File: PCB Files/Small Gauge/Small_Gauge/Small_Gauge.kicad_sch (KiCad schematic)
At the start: 30 parts, among them J1 USB_B_Micro, J2 Conn_01x02, J3 Conn_02x18_Odd_Even, J4 Conn_02x18_Odd_Even, U1 RP2040, U2 NCP1117-3.3_SOT223, U3 W25Q128JVS, Y1 ABM8G-12.000MHZ-18-D2Y-T3

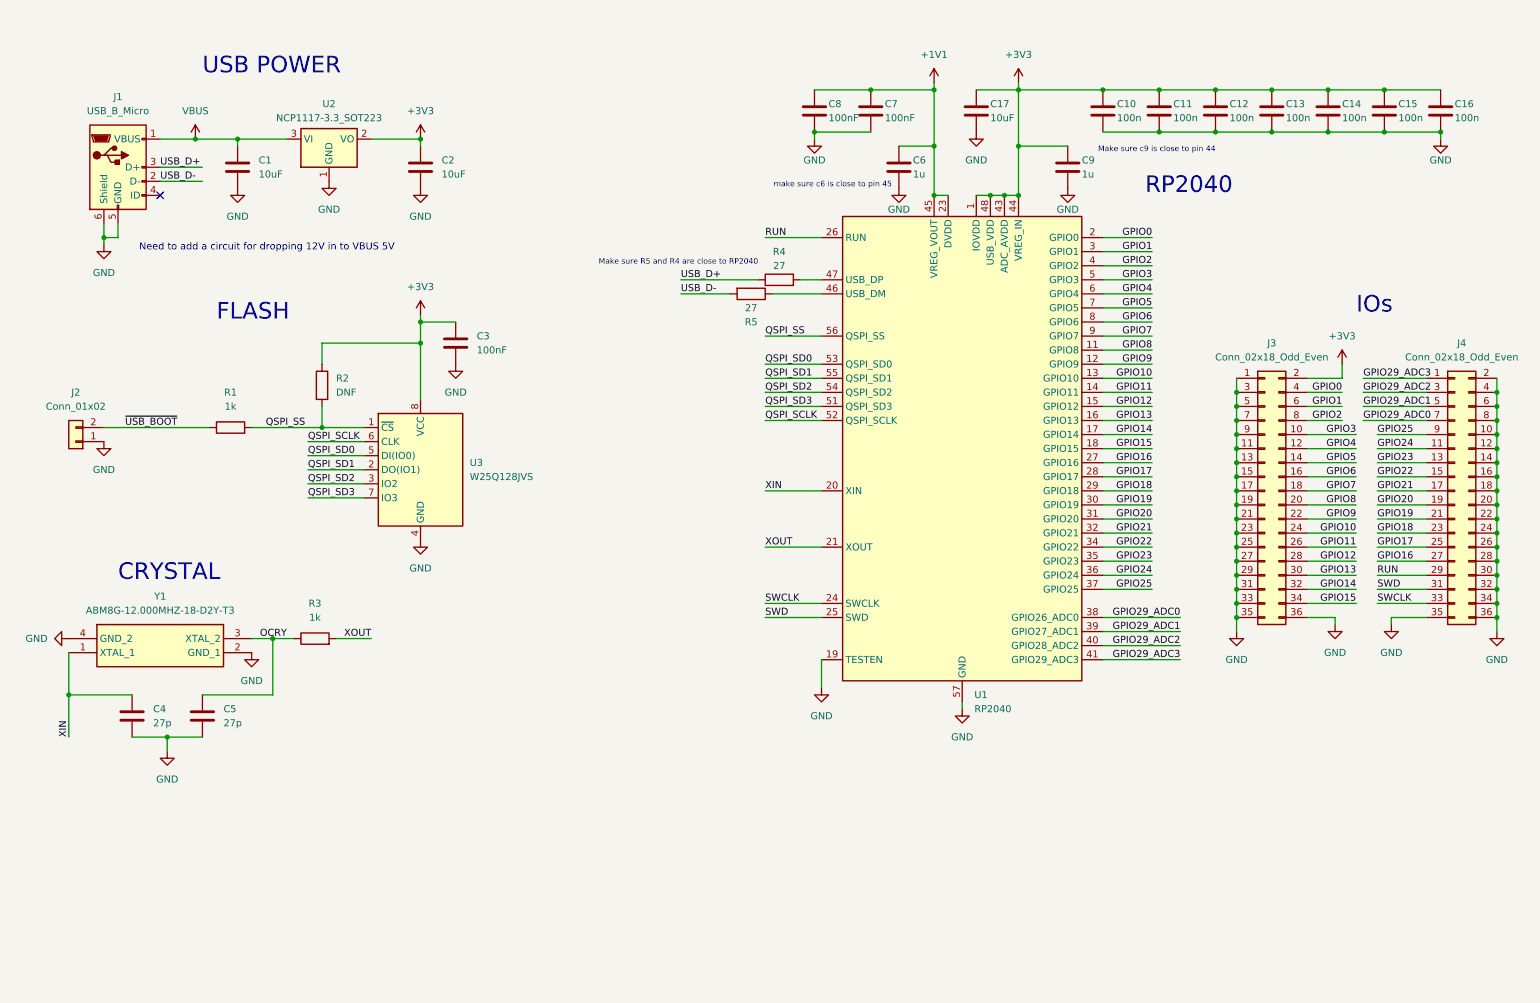
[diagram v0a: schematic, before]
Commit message: KiCad ESP 32 stuff
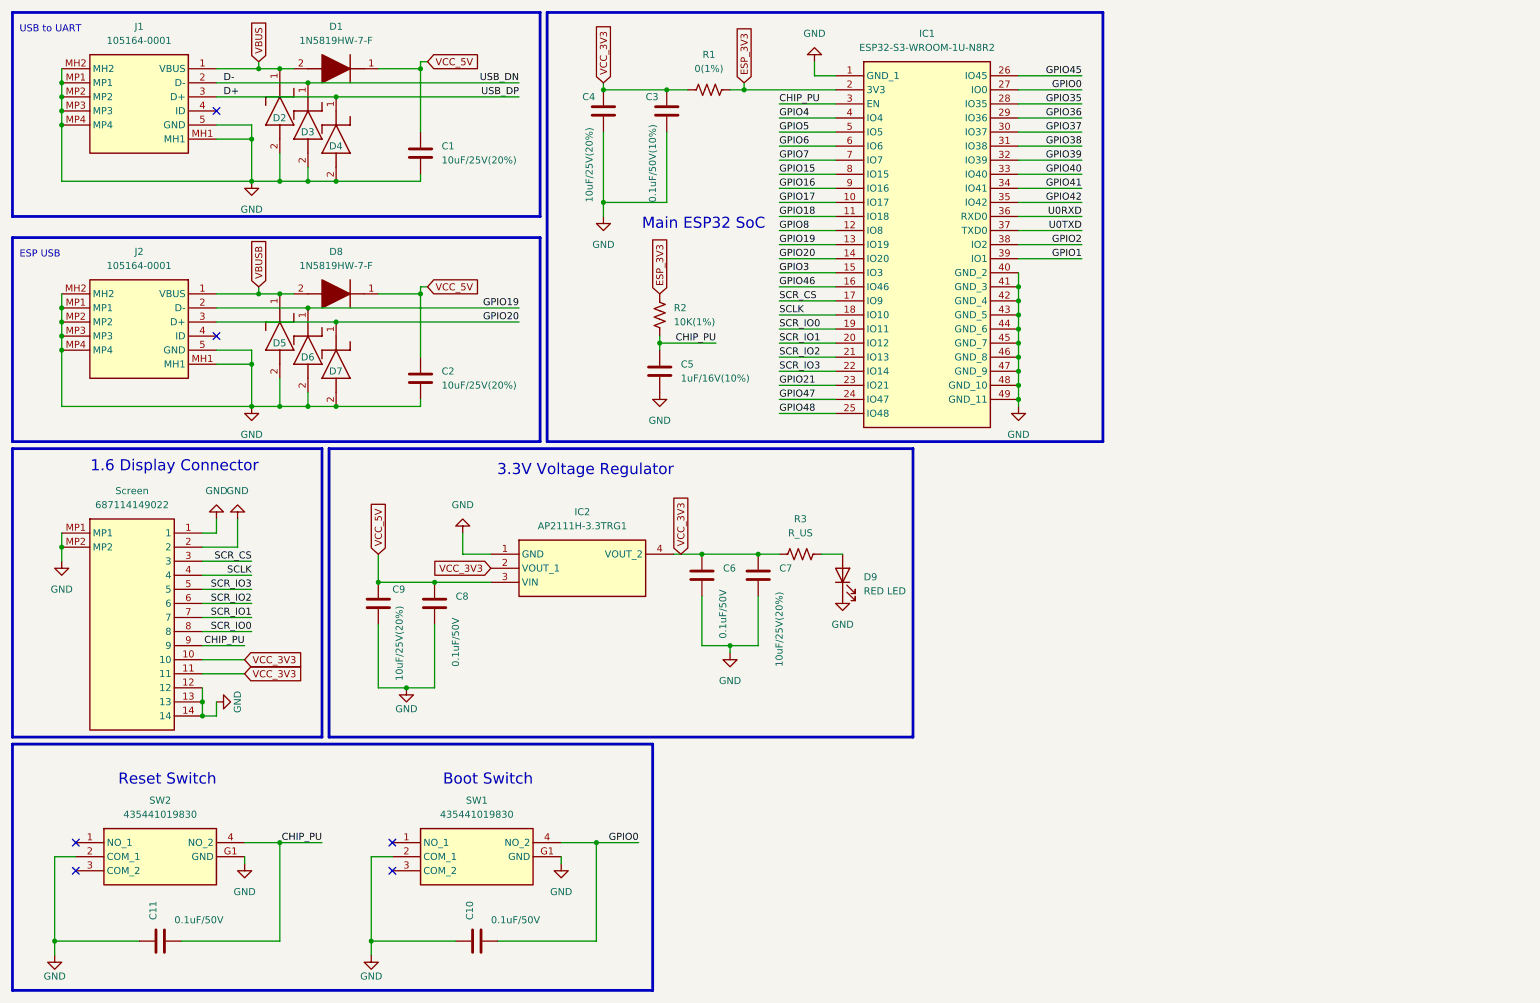
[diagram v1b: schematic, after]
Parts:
- removed C12, C13, C14, C15, C16: 100n, Resistor_SMD:R_0201_0603Metric, symbol Device:C
- removed C17: 10uF, Capacitor_SMD:C_0402_1005Metric_Pad0.74x0.62mm_HandSolder, symbol Device:C
- removed J1: USB_B_Micro, Mouser:USB_MICRO_B_1051640001, symbol Connector:USB_B_Micro
- removed J2: Conn_01x02, Connector_JST:JST_EH_B2B-EH-A_1x02_P2.50mm_Vertical, symbol Connector_Generic:Conn_01x02
- removed J3, J4: Conn_02x18_Odd_Even, Connector_JST:JST_PUD_B36B-PUDSS_2x18_P2.00mm_Vertical, symbol Connector_Generic:Conn_02x18_Odd_Even
- removed R1, R3: 1k, Resistor_SMD:R_0201_0603Metric_Pad0.64x0.40mm_HandSolder, symbol Device:R
- removed R2: DNF, Resistor_SMD:R_0201_0603Metric_Pad0.64x0.40mm_HandSolder, symbol Device:R
- removed R4, R5: 27, Resistor_SMD:R_0402_1005Metric, symbol Device:R
- removed U1: RP2040, Package_DFN_QFN:QFN-56-1EP_7x7mm_P0.4mm_EP3.2x3.2mm, symbol MCU_RaspberryPi:RP2040
- removed U2: NCP1117-3.3_SOT223, Package_TO_SOT_SMD:SOT-223-3_TabPin2, symbol Regulator_Linear:NCP1117-3.3_SOT223
- removed U3: W25Q128JVS, Package_SO:SOIC-8_5.23x5.23mm_P1.27mm, symbol Memory_Flash:W25Q128JVS
- removed Y1: ABM8G-12.000MHZ-18-D2Y-T3, Mouser:ABM8G, symbol ABM8G-12_000MHZ-18-D2Y-T3:ABM8G-12.000MHZ-18-D2Y-T3
- added D1, D8: 1N5819HW-7-F, SOD3716X145N, symbol SamacSys_Parts:1N5819HW-7-F
- added D2, D3, D4, D5, D6, D7: ESDA7P60-1U1M, ESDA7P601U1M, symbol SamacSys_Parts:ESDA7P60-1U1M
- added D9: RED LED, Resistor_SMD:R_1206_3216Metric_Pad1.30x1.75mm_HandSolder, symbol Device:LED
- added IC1: ESP32-S3-WROOM-1U-N8R2, ESP32S3WROOM1UN8R2, symbol SamacSys_Parts:ESP32-S3-WROOM-1U-N8R2
- added IC2: AP2111H-3.3TRG1, SOT230P700X180-4N, symbol SamacSys_Parts:AP2111H-3.3TRG1
- added J1, J2: 105164-0001, 1051640001, symbol SamacSys_Parts:105164-0001
- added R1: 0(1%), Resistor_SMD:R_0603_1608Metric_Pad0.98x0.95mm_HandSolder, symbol Device:R_US
- added R2: 10K(1%), Resistor_SMD:R_1206_3216Metric, symbol Device:R_US
- added R3: R_US, Resistor_SMD:R_1206_3216Metric, symbol Device:R_US
- added SW1, SW2: 435441019830, SamacSys_Parts:435441019830, symbol SamacSys_Parts:435441019830
- added Screen: 687114149022, 687114149022, symbol SamacSys_Parts:687114149022
- C1, C2: value 10uF -> 10uF/25V(20%); footprint Capacitor_SMD:C_0402_1005Metric_Pad0.74x0.62mm_HandSolder -> Capacitor_SMD:C_1206_3216Metric; Price 0.27 -> (none); Vendor https://www.mouser.com/ProductDetail/KYOCERA-AVX/04026D106M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 -> (none)
- C10, C11: value 100n -> 0.1uF/50V; footprint Resistor_SMD:R_0201_0603Metric -> Resistor_SMD:R_1206_3216Metric; Price 0.10 -> (none); Vendor https://www.mouser.com/ProductDetail/TDK/C0603X5R1E104K030B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 -> (none)
- C3: value 100nF -> 0.1uF/50V(10%); footprint Resistor_SMD:R_0201_0603Metric -> (none); Price 0.10 -> (none); Vendor https://www.mouser.com/ProductDetail/TDK/C0603X5R1E104K030B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 -> (none)
- C4: value 27p -> 10uF/25V(20%); footprint Capacitor_SMD:C_0201_0603Metric -> (none); Price 0.10 -> (none); Vendor https://www.mouser.com/ProductDetail/Murata-Electronics/GRT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 -> (none)
- C5: value 27p -> 1uF/16V(10%); footprint Capacitor_SMD:C_0201_0603Metric -> Resistor_SMD:R_1206_3216Metric; Price 0.10 -> (none); Vendor https://www.mouser.com/ProductDetail/Murata-Electronics/GRT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 -> (none)
- C6: value 1u -> 0.1uF/50V; footprint Capacitor_SMD:C_0201_0603Metric -> Resistor_SMD:R_1206_3216Metric; Price 0.12 -> (none); Vendor https://www.mouser.com/ProductDetail/KYOCERA-AVX/02016D105M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 -> (none)
- C7: value 100nF -> 10uF/25V(20%); footprint Resistor_SMD:R_0201_0603Metric -> Resistor_SMD:R_1206_3216Metric; Price 0.10 -> (none); Vendor https://www.mouser.com/ProductDetail/TDK/C0603X5R1E104K030B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 -> (none)
- C8: value 100nF -> 0.1uF/50V; footprint Resistor_SMD:R_0201_0603Metric -> Resistor_SMD:R_1206_3216Metric; Price 0.10 -> (none); Vendor https://www.mouser.com/ProductDetail/TDK/C0603X5R1E104K030B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 -> (none)
- C9: value 1u -> 10uF/25V(20%); footprint Capacitor_SMD:C_0201_0603Metric -> Resistor_SMD:R_1206_3216Metric; Price 0.12 -> (none); Vendor https://www.mouser.com/ProductDetail/KYOCERA-AVX/02016D105M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 -> (none)
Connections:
- net XIN is gone; now on net VCC_3V3: C4.1
- net GND: now also C10.1, C11.1, D2.2 (A), D3.2 (A), D4.2 (A), D5.2 (A), D6.2 (A), D7.2 (A), D9.1 (K), IC1.1 (GND_1), IC1.40 (GND_2), IC1.41 (GND_3), IC1.42 (GND_4), IC1.43 (GND_5), IC1.44 (GND_6), IC1.45 (GND_7), IC1.46 (GND_8), IC1.47 (GND_9), IC1.48 (GND_10), IC1.49 (GND_11), IC2.1 (GND), J1.5 (GND), J1.MH1, J1.MH2, J1.MP1, J1.MP2, J1.MP3, J1.MP4, J2.5 (GND), J2.MH1, J2.MH2, J2.MP1, J2.MP2, J2.MP3, J2.MP4, SW1.2 (COM_1), SW1.G1 (GND), SW2.2 (COM_1), SW2.G1 (GND), Screen.1, Screen.12, Screen.13, Screen.14, Screen.2, Screen.MP1, Screen.MP2; no longer C10.2, C11.2
- net GPIO0: now also C10.2, IC1.27 (IO0), SW1.4 (NO_2)
- net GPIO1: now also IC1.39 (IO1)
- net GPIO15: now also IC1.8 (IO15)
- net GPIO16: now also IC1.9 (IO16)
- net GPIO17: now also IC1.10 (IO17)
- net GPIO18: now also IC1.11 (IO18)
- net GPIO19: now also D6.1 (K), IC1.13 (IO19), J2.2 (D-)
- net GPIO2: now also IC1.38 (IO2)
- net GPIO20: now also D7.1 (K), IC1.14 (IO20), J2.3 (D+)
- net GPIO21: now also IC1.23 (IO21)
- net GPIO3: now also IC1.15 (IO3)
- net GPIO4: now also IC1.4 (IO4)
- net GPIO5: now also IC1.5 (IO5)
- net GPIO6: now also IC1.6 (IO6)
- net GPIO7: now also IC1.7 (IO7)
- net GPIO8: now also IC1.12 (IO8)
- net VBUS: now also D1.2 (A), D2.1 (K), J1.1 (VBUS); no longer C1.1
- net +1V1 renamed VCC_3V3
- net VCC_3V3: now also C3.1, IC2.2 (VOUT_1), IC2.4 (VOUT_2), R1.1, R3.1, Screen.10, Screen.11; no longer C8.1
- removed net +3V3: C10.1, C11.1, C2.1, C3.1, C9.1
- net OCRY renamed CHIP_PU
- net CHIP_PU: now also C11.2, IC1.3 (EN), R2.2, SW2.4 (NO_2), Screen.9
- new net: D9.2 (A), R3.2
- new net D+: D4.1 (K), J1.3 (D+)
- new net D-: D3.1 (K), J1.2 (D-)
- new net ESP_3V3: IC1.2 (3V3), R1.2, R2.1
- new net GPIO35: IC1.28 (IO35)
- new net GPIO36: IC1.29 (IO36)
- new net GPIO37: IC1.30 (IO37)
- new net GPIO38: IC1.31 (IO38)
- new net GPIO39: IC1.32 (IO39)
- new net GPIO40: IC1.33 (IO40)
- new net GPIO41: IC1.34 (IO41)
- new net GPIO42: IC1.35 (IO42)
- new net GPIO45: IC1.26 (IO45)
- new net GPIO46: IC1.16 (IO46)
- new net GPIO47: IC1.24 (IO47)
- new net GPIO48: IC1.25 (IO48)
- new net SCLK: IC1.18 (IO10), Screen.4
- new net SCR_CS: IC1.17 (IO9), Screen.3
- new net SCR_IO0: IC1.19 (IO11), Screen.8
- new net SCR_IO1: IC1.20 (IO12), Screen.7
- new net SCR_IO2: IC1.21 (IO13), Screen.6
- new net SCR_IO3: IC1.22 (IO14), Screen.5
- new net U0RXD: IC1.36 (RXD0)
- new net U0TXD: IC1.37 (TXD0)
- new net VBUSB: D5.1 (K), D8.2 (A), J2.1 (VBUS)
- new net VCC_5V: C1.1, C2.1, C8.1, C9.1, D1.1 (K), D8.1 (K), IC2.3 (VIN)
- no-connect marks 1 -> 6
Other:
- note added: "1.6 Display Connector"
- note added: "3.3V Voltage Regulator"
- note added: "Boot Switch"
- note added: "ESP USB"
- note added: "Main ESP32 SoC"
- note added: "Reset Switch"
- note added: "USB to UART"
- note removed: "CRYSTAL"
- note removed: "FLASH"
- note removed: "IOs"
- note removed: "Make sure R5 and R4 are close to RP2040"
- note removed: "Make sure c9 is close to pin 44"
- note removed: "Need to add a circuit for dropping 12V in to VBUS 5V"
- note removed: "RP2040"
- note removed: "USB POWER"
- note removed: "make sure c6 is close to pin 45"
